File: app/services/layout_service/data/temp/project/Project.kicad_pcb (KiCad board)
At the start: 2 copper layers, 48 x 48 mm, 22 parts, among them J1 ASSMANN_AU-Y1007, U1 SOT-23_MC_MCH, U2 QFN40P300X300X90-21N, X1 CRYSTAL_ABM8G_ABR

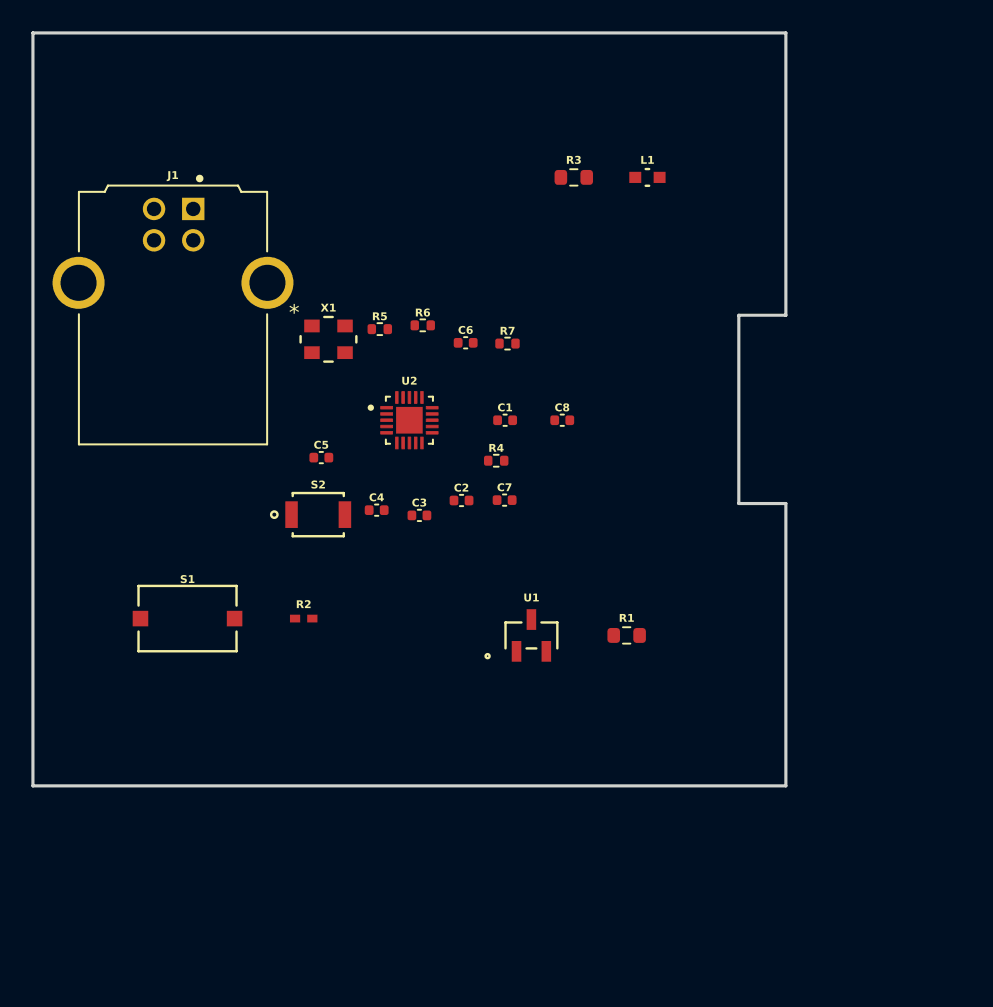
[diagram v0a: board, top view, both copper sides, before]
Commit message: 动态适配本地板子-2.2
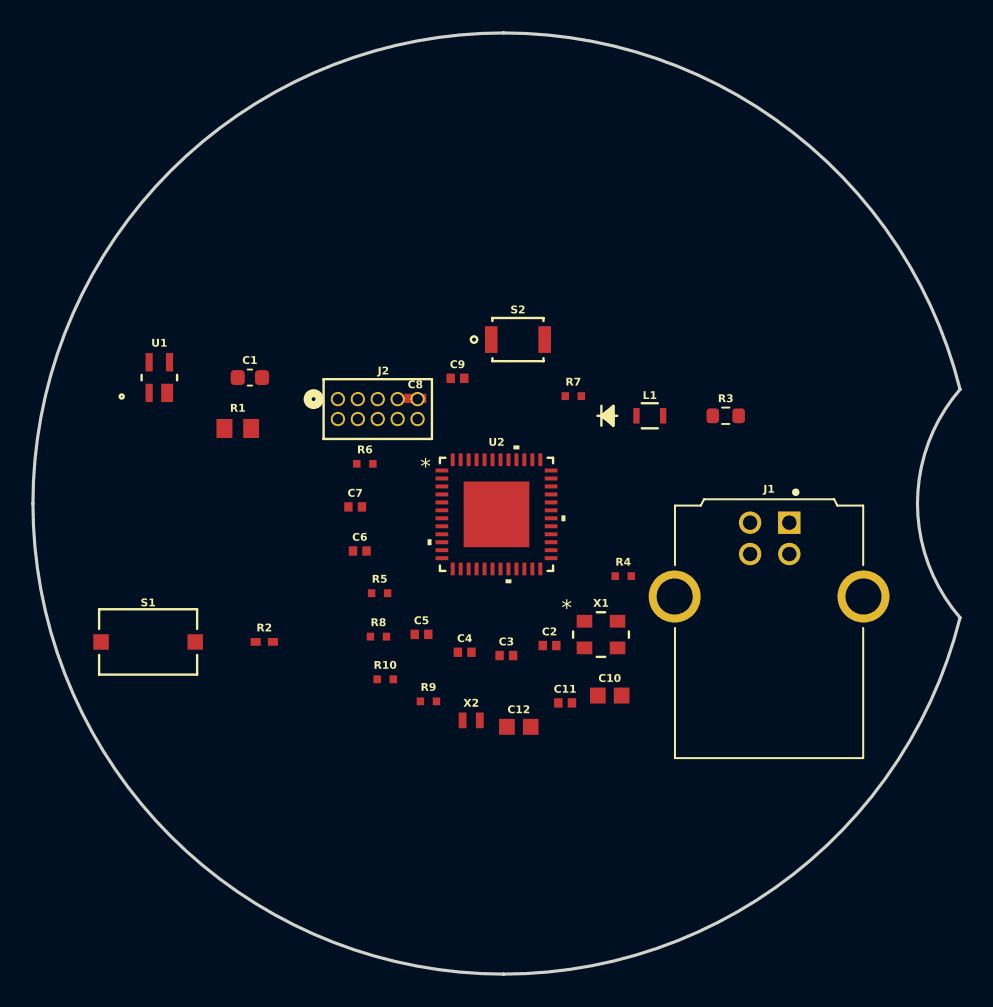
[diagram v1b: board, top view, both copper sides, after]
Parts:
- added C10: CAPC1608X100N, 0603C, F.Cu at (161.8, 112.2)
- added C11: CAPC1005X55N, 0402C, F.Cu at (158.9, 112.7)
- added C12: CAPC1608X100N, 0603C, F.Cu at (156.0, 114.2)
- added C9: CAPC1005X55N, 0402C, F.Cu at (152.1, 92.0)
- added J2: CONN10_500542_HRW, M50_3500542, F.Cu at (144.4, 93.3)
- added R10: RES_ERJ-2GEJ103X, 0402R, F.Cu at (147.5, 111.2)
- added R8: RES_ERJ-2GEJ103X, 0402R, F.Cu at (147.0, 108.5)
- added R9: RES_ERJ-2GEJ103X, 0402R, F.Cu at (150.2, 112.6)
- added X2: XTAL_ABS05-32.768KHZ-T, ABS05_32_768KHZ_T, F.Cu at (152.9, 113.8)
- C1: value C_0402_1005Metric -> C_0603_1608Metric; footprint C_0402_1005Metric -> C_0603_1608Metric
- C2, C3, C4, C5, C6, C7, C8: value C_0402_1005Metric -> CAPC1005X55N; footprint C_0402_1005Metric -> 0402C
- L1: value LED_LTST-C191KRKT_LTO -> LED_GS75000_WRE; footprint LED_LTST-C191KRKT_LTO -> LED_GS75000_WRE
- R1: value R_0603_1608Metric -> RC0805N_YAG; footprint R_0603_1608Metric -> RC0805N_YAG
- R4, R5, R6, R7: value R_0402_1005Metric -> RES_ERJ-2GEJ103X; footprint R_0402_1005Metric -> 0402R
- U1: value SOT-23_MC_MCH -> 21-0098_X4+1_MXM; footprint SOT-23_MC_MCH -> 21-0098_X4&plus_1_MXM
- U2: value QFN40P300X300X90-21N -> QFN48_7X7MC_MCH; footprint QFN40P300X300X90-21N -> QFN48_7X7MC_MCH
- moved J1 42.9 mm to (171.9, 108.0)
- moved U1 28.9 mm to (133.1, 92.0)
- moved R1 28.1 mm to (138.1, 95.2)
- moved X1 25.6 mm to (161.2, 108.4)
- moved R3 18.0 mm to (169.2, 94.4)
- moved S2 16.9 mm to (155.9, 89.5)
- moved R5 16.8 mm to (147.1, 105.7)
- moved C1 16.5 mm to (138.8, 92.0)
- moved L1 15.2 mm to (164.3, 94.4)
- moved C6 14.9 mm to (145.8, 103.0)
- moved C5 13.0 mm to (149.8, 108.3)
- moved R4 10.9 mm to (162.6, 104.6)
- moved C2 10.8 mm to (157.9, 109.1)
- moved C4 10.7 mm to (152.5, 109.5)
- moved C3 10.5 mm to (155.2, 109.7)
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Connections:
- net Net-(R3-2) renamed KLT_3_PA06
- C1 pad 1: Net-(C6-1) -> Net-(C1-Pad1)
- C1 pad 2: Net-(C6-2) -> unconnected-(C1--Pad2)
- C2 pad 1: Net-(C6-1) -> Net-(X1-OUT/IN)
- C2 pad 2: Net-(C6-2) -> Net-(C2-2)
- C3 pad 1: Net-(C6-1) -> Net-(C5-1)
- C3 pad 2: Net-(C6-2) -> Net-(C3-2)
- C4 pad 1: Net-(R5-1) -> Net-(C5-1)
- C4 pad 2: Net-(C4-2) -> Net-(C3-2)
- C5 pad 2: Net-(C5-2) -> Net-(C3-2)
- C6 pad 1: Net-(C6-1) -> KLT_1_XIN32
- C7 pad 1: Net-(U2-PB2(TOSC2)) -> Net-(X1-IN/OUT)
- C8 pad 1: Net-(C6-1) -> Net-(C8-1)
- C8 pad 2: Net-(C6-2) -> Net-(C8-2)
- J1 pad 2: KLT_4_PC1 -> KLT_5_PA08
- J1 pad 3: KLT_3_PB4 -> KLT_4_PA07
- L1 pad 1: unconnected-(L1--Pad1) -> Net-(L1-Pad1)
- R1 pad 1: KLT_1_PA7 -> KLT_1_XIN32
- R2 pad 1: KLT_2_PA2 -> KLT_2_PA05
- R4 pad 1: Net-(U2-PB0) -> Net-(R4-1)
- R5 pad 2: Net-(S2-2) -> Net-(R5-2)
- R6 pad 1: Net-(R5-1) -> Net-(U2-PA22)
- R7 pad 1: Net-(R7-1) -> Net-(U2-PA17)
- S1 pad 2: KLT_2_PA2 -> KLT_2_PA05
- U1 pad 3: KLT_1_PA7 -> Net-(C1-Pad1)
- U2 pad 1: KLT_2_PA2 -> (no net)
- U2 pad 10: KLT_3_PB4 -> (no net)
- U2 pad 11: Net-(C5-1) -> (no net)
- U2 pad 12: Net-(U2-PB2(TOSC2)) -> (no net)
- U2 pad 13: Net-(R7-1) -> (no net)
- U2 pad 14: Net-(U2-PB0) -> (no net)
- U2 pad 15: Net-(U2-PC0) -> (no net)
- U2 pad 16: KLT_4_PC1 -> (no net)
- U2 pad 17: Net-(U2-PC2) -> (no net)
- U2 pad 18: Net-(U2-PC3) -> (no net)
- U2 pad 19: Net-(R5-1) -> (no net)
- U2 pad 2: Net-(U2-PA3(EXTCLK)) -> (no net)
- U2 pad 20: Net-(U2-PA1) -> (no net)
- U2 pad 21: unconnected-(U2-EXP-Pad21) -> (no net)
- U2 pad 3: Net-(U2-GND) -> (no net)
- U2 pad 4: Net-(U2-VDD) -> (no net)
- U2 pad 5: Net-(U2-PA4) -> (no net)
- U2 pad 6: Net-(U2-PA5) -> (no net)
- U2 pad 7: Net-(U2-PA6) -> (no net)
- U2 pad 8: KLT_1_PA7 -> (no net)
- U2 pad 9: Net-(U2-PB5) -> (no net)
- X1 pad 1: Net-(C5-1) -> Net-(X1-IN/OUT)
- X1 pad 3: Net-(U2-PB2(TOSC2)) -> Net-(X1-OUT/IN)
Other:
- board size 48 x 48 mm -> 59.1 x 60 mm
